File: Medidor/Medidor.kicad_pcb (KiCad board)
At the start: 2 copper layers, 79 x 43.8 mm, 45 parts, among them J1 TC2030-CTX-TAG_CONECT, SW1 Rotary_Encoder_Switch, SW2 SW_DPST_x2, U1 INA219-INA, U3 2450AT18D0100, X1 32MHz

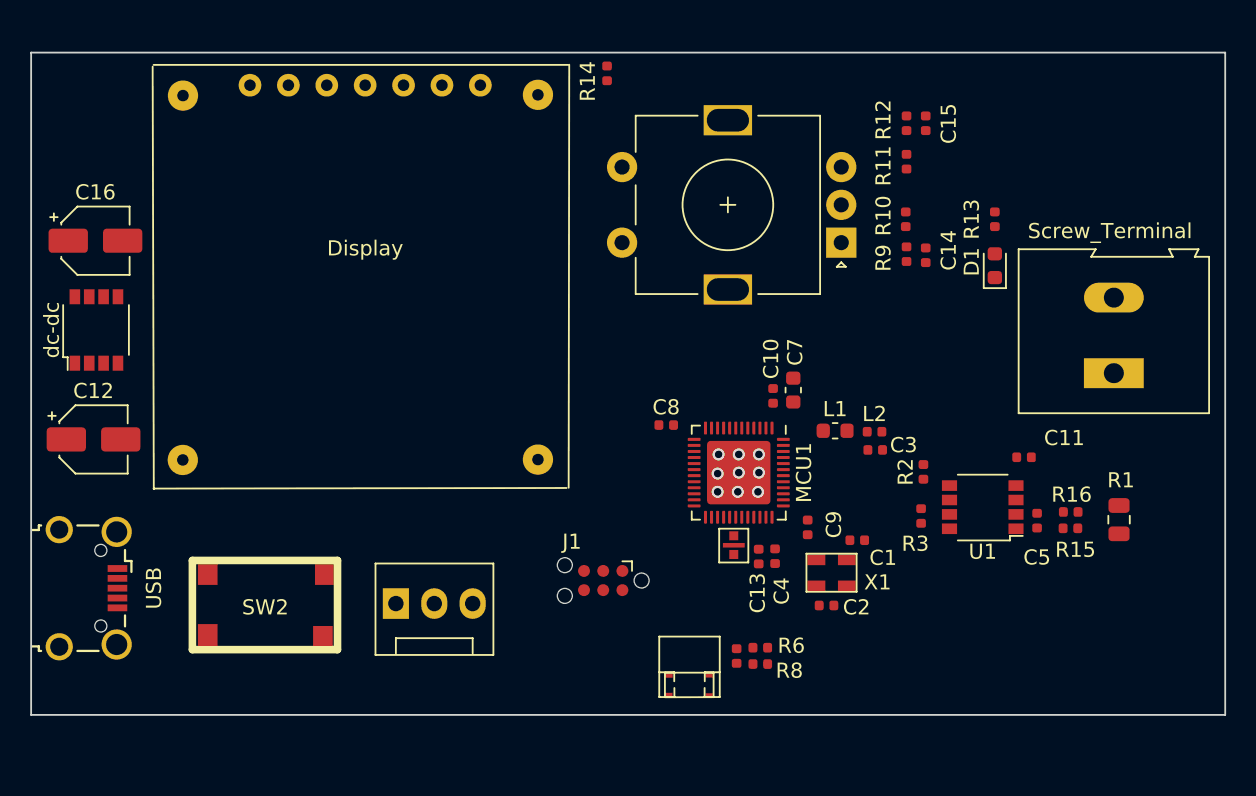
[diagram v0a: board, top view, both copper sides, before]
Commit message: Add files via upload
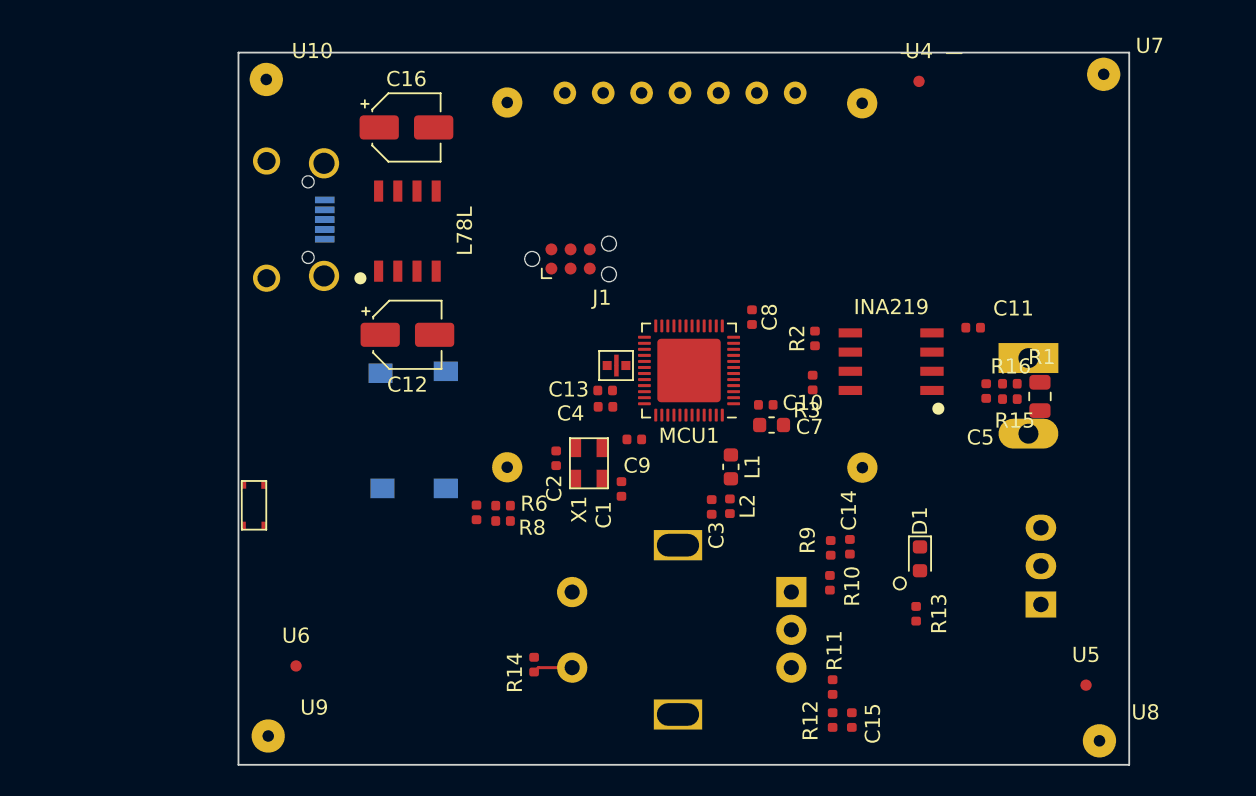
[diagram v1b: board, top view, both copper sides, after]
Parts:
- removed U1: INA219-INA, Package_TO_SOT_SMD:SuperSOT-8
- removed dc-dc: DC-DC, Package_TO_SOT_SMD:SuperSOT-8
- added  L78L: L78L, Medidor:L78L, F.Cu at (94.7, 100.1)
- added INA219: INA219, Medidor:INA219, F.Cu at (126.7, 108.7)
- added U10: spacer, Medidor:spacer, F.Cu at (85.5, 90.4)
- added U4: Fiducial, Fiducial:Fiducial_0.75mm_Mask1.5mm, F.Cu at (128.6, 90.2)
- added U5: Fiducial, Fiducial:Fiducial_0.75mm_Mask1.5mm, F.Cu at (139.6, 130.1)
- added U6: Fiducial, Fiducial:Fiducial_0.75mm_Mask1.5mm, F.Cu at (87.4, 128.8)
- added U7: spacer, Medidor:spacer, F.Cu at (140.9, 90.1)
- added U8: spacer, Medidor:spacer, F.Cu at (140.6, 134.2)
- added U9: spacer, Medidor:spacer, F.Cu at (85.6, 133.9)
- Display, SW1, SW2, Screw_Terminal, USB: moved to B.Cu
- U2: renamed from UART; moved to B.Cu
- moved U2 42.7 mm to (136.7, 124.8), turned to 90 degrees
- moved C15 39.8 mm to (124.1, 132.4), turned to 270 degrees
- moved R12 39.8 mm to (122.9, 132.4), turned to 90 degrees
- moved R14 39.4 mm to (103.1, 128.8)
- moved R11 35.1 mm to (122.9, 130.2), turned to 270 degrees
- moved U3 31.1 mm to (85.4, 119.8), turned to 90 degrees
- moved USB 28.0 mm to (87.4, 99.3), turned to 90 degrees
- moved R13 26.6 mm to (128.4, 125.4), turned to 270 degrees
- moved R10 24.6 mm to (122.7, 123.3), turned to 270 degrees
- moved SW1 23.3 mm to (120.1, 124.0)
- moved C16 21.9 mm to (94.7, 93.2)
- moved C12 21.9 mm to (94.7, 106.9)
- moved J1 21.4 mm to (105.5, 101.9), turned to 0 degrees
- moved Display 20.8 mm to (112.8, 103.6), turned to 180 degrees
- moved C2 20.4 mm to (104.6, 115.1), turned to 90 degrees
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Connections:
- MCU1 pad 15: /TX -> Net-(MCU1-Pad15)
- MCU1 pad 16: /RX -> Net-(MCU1-Pad16)
- MCU1 pad 3: Net-(MCU1-Pad3) -> /TX
- MCU1 pad 38: Net-(MCU1-Pad38) -> RC1
- MCU1 pad 39: Net-(MCU1-Pad39) -> RC2
- MCU1 pad 4: RC3 -> /RX
- MCU1 pad 42: SDA -> LEDMCU
- MCU1 pad 43: SCL -> RC3
- MCU1 pad 5: RC2 -> Net-(MCU1-Pad5)
- MCU1 pad 6: RC1 -> Net-(MCU1-Pad6)
- MCU1 pad 8: LEDMCU -> SDA
- MCU1 pad 9: Net-(MCU1-Pad9) -> SCL
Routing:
- net RC3: track 0.00 -> 2.64 mm
- net GND: vias 9 -> 0
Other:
- board size 79 x 43.8 mm -> 58.9 x 47.1 mm
